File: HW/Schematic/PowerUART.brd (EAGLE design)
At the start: 29.1 x 35.4 mm, 62 parts, among them U2 CP2104QFN_PAD

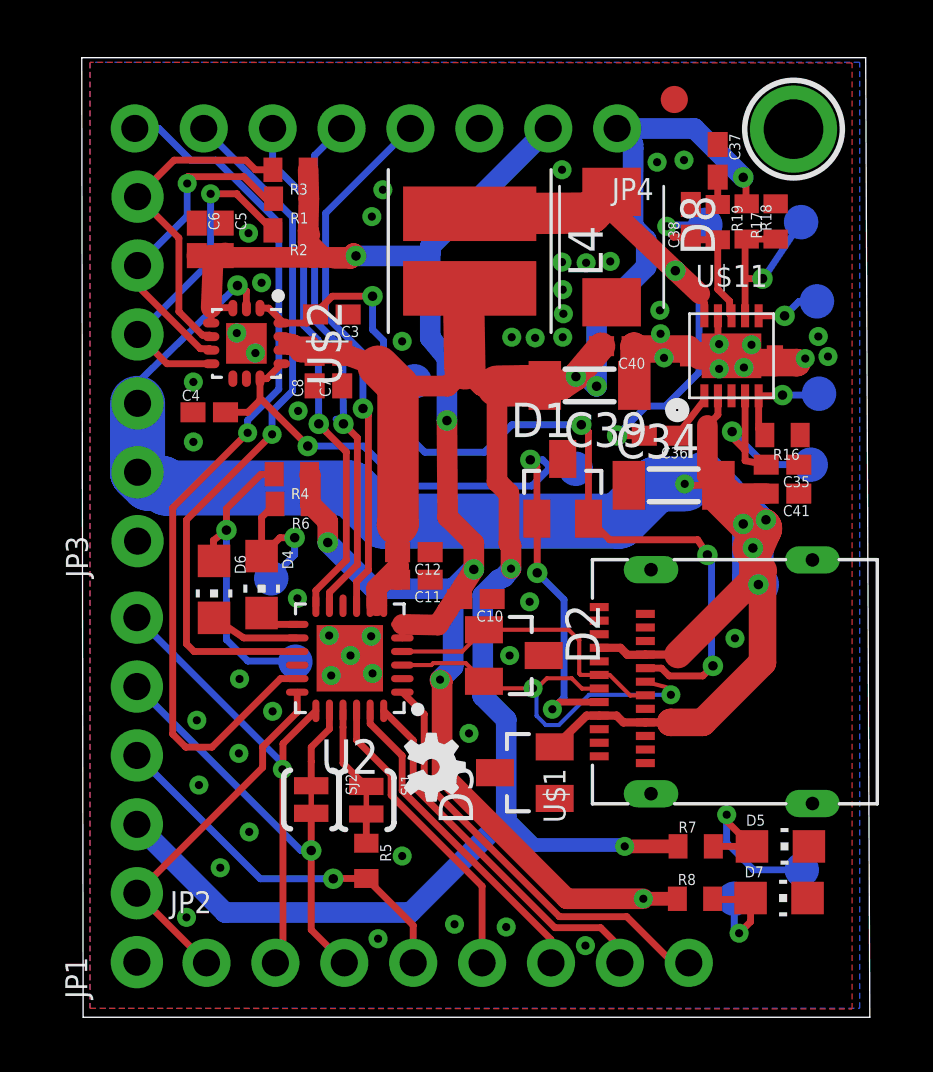
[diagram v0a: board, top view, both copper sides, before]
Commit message: add testpoints.csv
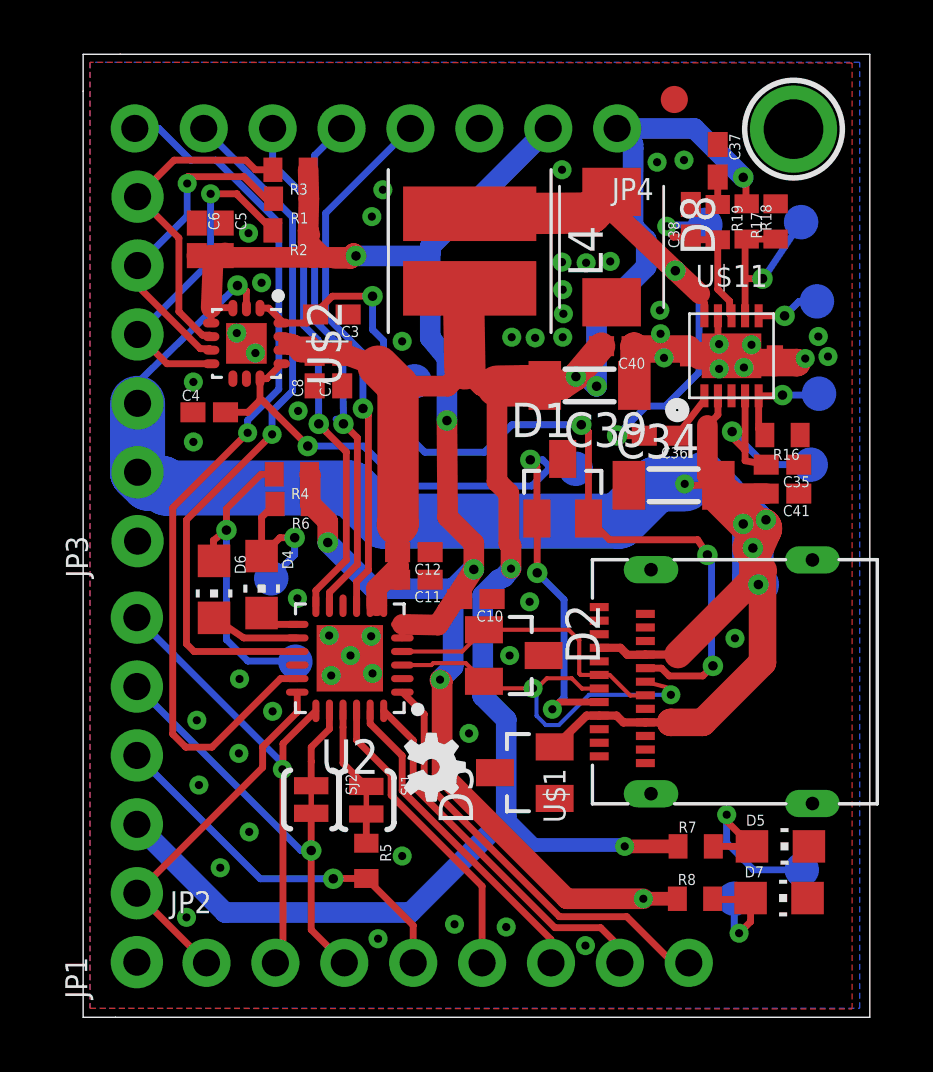
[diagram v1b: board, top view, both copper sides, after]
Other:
- board size 29.1 x 35.4 mm -> 29 x 35.5 mm
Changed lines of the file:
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@@
 <setting verticaltext="up"/>
 </settings>
-<grid distance="1" unitdist="mil" unit="mil" style="lines" multiple="1" display="yes" altdistance="0.000123031496" altunitdist="mil" altunit="mil"/>
+<grid distance="1" unitdist="mil" unit="mm" style="lines" multiple="1" display="yes" altdistance="0.000123031496" altunitdist="mil" altunit="mil"/>
 <layers>
 <layer number="1" name="Top" color="4" fill="1" visible="yes" active="yes"/>
@@
 <fusionsync huburn="a.cGVyc29uYWw6dWUyOTdhZGZi" projecturn="a.cGVyc29uYWw6dWUyOTdhZGZiIzIwMTYwMTA4MjIzOTY3MjY" f3durn="urn:adsk.wipprod:dm.lineage:jQXCEEFlSgyEhEQMhi0FtQ" pcbguid="53d00ac5-8cbc-41ab-bffd-7753b437712b" lastpulledtime="" lastsyncedchangeguid="e1987d31-fde6-4ada-60cd-040e15f8273c"/>
 <plain>
-<wire x1="0" y1="0" x2="29" y2="0" width="0" layer="20"/>
-<wire x1="29" y1="0" x2="28.8476" y2="35.3736" width="0" layer="20"/>
-<wire x1="28.8476" y1="35.3736" x2="-0.0508" y2="35.3736" width="0" layer="20"/>
-<wire x1="-0.0508" y1="35.3736" x2="0" y2="0" width="0" layer="20"/>
+<wire x1="0" y1="0" x2="1.1938" y2="0" width="0" layer="20"/>
+<wire x1="1.1938" y1="0" x2="29" y2="0" width="0" layer="20"/>
+<wire x1="29" y1="0" x2="29" y2="35.5" width="0" layer="20"/>
+<wire x1="29" y1="35.5" x2="0" y2="35.5" width="0" layer="20"/>
+<wire x1="0" y1="35.5" x2="0" y2="34.1376" width="0" layer="20"/>
 <text x="25.1968" y="27.3558" size="1.27" layer="38" font="vector" rot="MR270">Engineerd by
 @bindebende
@@
 <text x="3.2258" y="29.7434" size="1.016" layer="26" font="vector" rot="MR180">/INT</text>
 <text x="3.113153125" y="32.11484375" size="1.016" layer="26" font="vector" rot="MR225">SUS</text>
+<wire x1="0" y1="34.1376" x2="0" y2="1.1938" width="0" layer="20"/>
+<wire x1="0" y1="1.1938" x2="0" y2="0" width="0" layer="20"/>
 <wire x1="5.7912" y1="31.5214" x2="5.8166" y2="31.496" width="0.254" layer="26"/>
 <text x="3.2004" y="34.9504" size="1.016" layer="26" font="vector" rot="MR180">/SUS</text>
@@
 <wire x1="6.985" y1="23.7744" x2="4.572" y2="23.7744" width="0.254" layer="26"/>
 <text x="8.9154" y="18.8976" size="1.016" layer="26" font="vector" rot="MR90">20V 5A max</text>
+<wire x1="1.362696875" y1="35.500296875" x2="1.365834375" y2="35.500296875" width="0.000003125" layer="20"/>
 </plain>
 <attributes>
